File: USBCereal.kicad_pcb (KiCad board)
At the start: 2 copper layers, 24.3 x 19.6 mm, 15 parts, among them J1 USB_C, J2 Conn_01x06, U1 XC6206P332MR, U2 CH340C

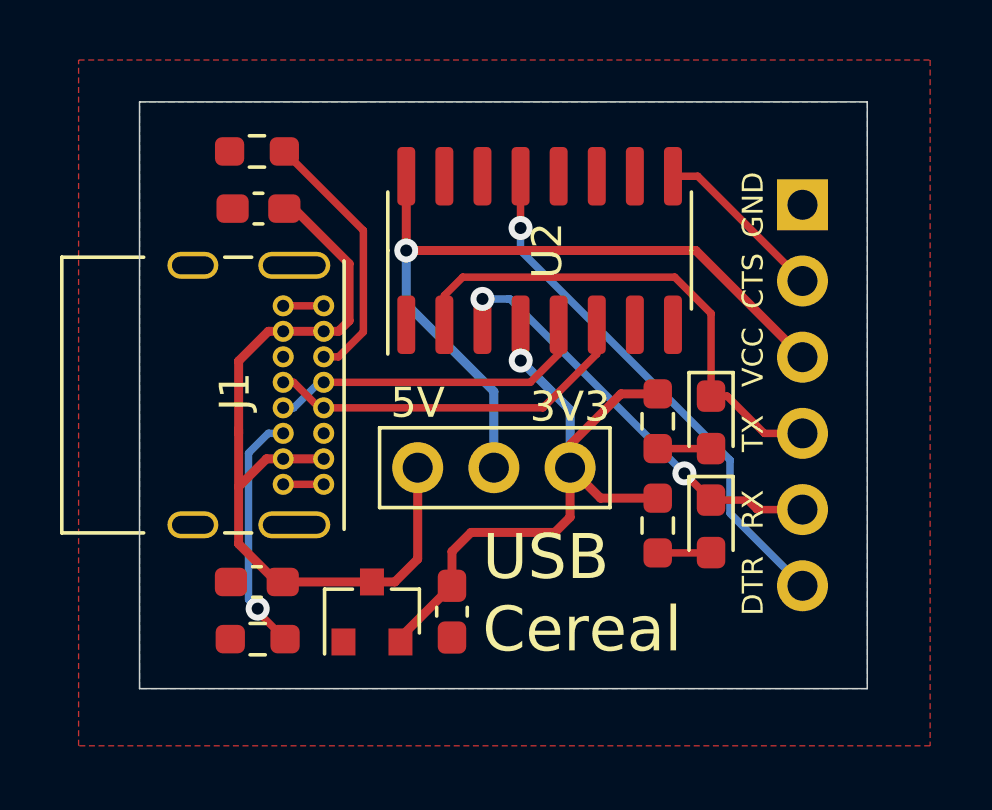
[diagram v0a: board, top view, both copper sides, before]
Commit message: Finished PCB, generated fabrication files
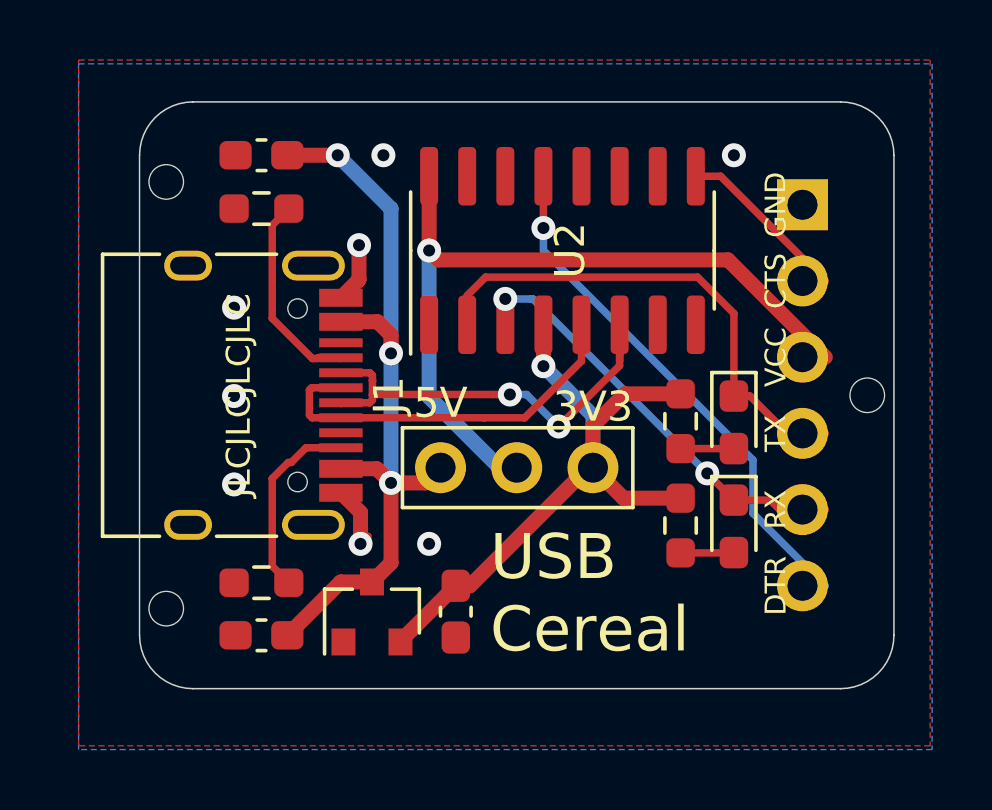
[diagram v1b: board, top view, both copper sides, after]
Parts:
- added REF**: JLCPCB_Tooling_Hole, USBCereal:JLCPCB_Tooling_Hole, F.Cu at (45.3, 27.1)
- added REF**: JLCPCB_Tooling_Hole, USBCereal:JLCPCB_Tooling_Hole, F.Cu at (22.0, 34.2)
- added REF**: JLCPCB_Tooling_Hole, USBCereal:JLCPCB_Tooling_Hole, F.Cu at (22.0, 19.9)
- J1: footprint Connector_USB:USB_C_Receptacle_GCT_USB4085 -> Connector_USB:USB_C_Receptacle_HRO_TYPE-C-31-M-12
- R3, R4: value 51 -> 47R
- moved J1 4.58 mm to (23.7, 27.1)
- moved R2 1.91 mm to (25.1, 20.8)
- moved R1 1.88 mm to (25.1, 33.3)
- moved C2 1.78 mm to (25.1, 35.1)
- moved C1 1.78 mm to (25.1, 19.1)
- moved G*** 1.76 mm to (35.8, 22.9)
- moved D1 0.76 mm to (40.9, 28.0)
- moved D2 0.76 mm to (40.9, 31.4)
- moved R3 0.76 mm to (39.1, 27.9)
- moved R4 0.76 mm to (39.1, 31.4)
- moved U2 0.76 mm to (35.2, 22.2)
- moved JP1 0.76 mm to (31.1, 29.5)
- moved C3 0.13 mm to (31.6, 34.3)
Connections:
- J1 pad A8: Net-(J1-PadA8) -> (no net)
- J1 pad B8: Net-(J1-PadB8) -> (no net)
- U2 pad 10: Net-(U2-Pad10) -> (no net)
- U2 pad 11: Net-(U2-Pad11) -> (no net)
- U2 pad 12: Net-(U2-Pad12) -> (no net)
- U2 pad 14: Net-(U2-Pad14) -> (no net)
- U2 pad 15: Net-(U2-Pad15) -> (no net)
- U2 pad 7: Net-(U2-Pad7) -> (no net)
- U2 pad 8: Net-(U2-Pad8) -> (no net)
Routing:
- net /USB_D-: track 12.5 -> 16.2 mm, vias 0 -> 2
- net /USB_D+: track 10.9 -> 13.0 mm
- net /CC1: track 8.77 -> 6.78 mm
- net +5V: track 29.0 -> 27.1 mm, vias 0 -> 3
- net /CC2: track 8.13 -> 6.42 mm, vias 1 -> 0
- net GNDD: track 2.70 -> 4.34 mm, vias 0 -> 8
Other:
- board size 24.3 x 19.6 mm -> 25.1 x 19.6 mm
- net class VCC: trace_width 0.3 -> 0.5
- board text added: "JLCJLCJLCJLC"
